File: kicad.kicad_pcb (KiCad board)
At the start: 2 copper layers, 100 x 70 mm, 65 parts, among them J1 Conn_01x03, J2 Screw_Terminal_01x02, J3 Conn_01x05, J4 jack3.5mm, J5 Screw_Terminal_01x02, J6 ICSP, J7 Screw_Terminal_01x03, J8 Screw_Terminal_01x03, K1 RELAY 0510, K2 RELAY 0510, Q1 BC817, Q2 BC817, SW1 SW_Push, SW2 SW_Push, T1 ZMPT101B, U1 KF33BD-TR, U2 ADS1015IDGS, U3 ESP-12E

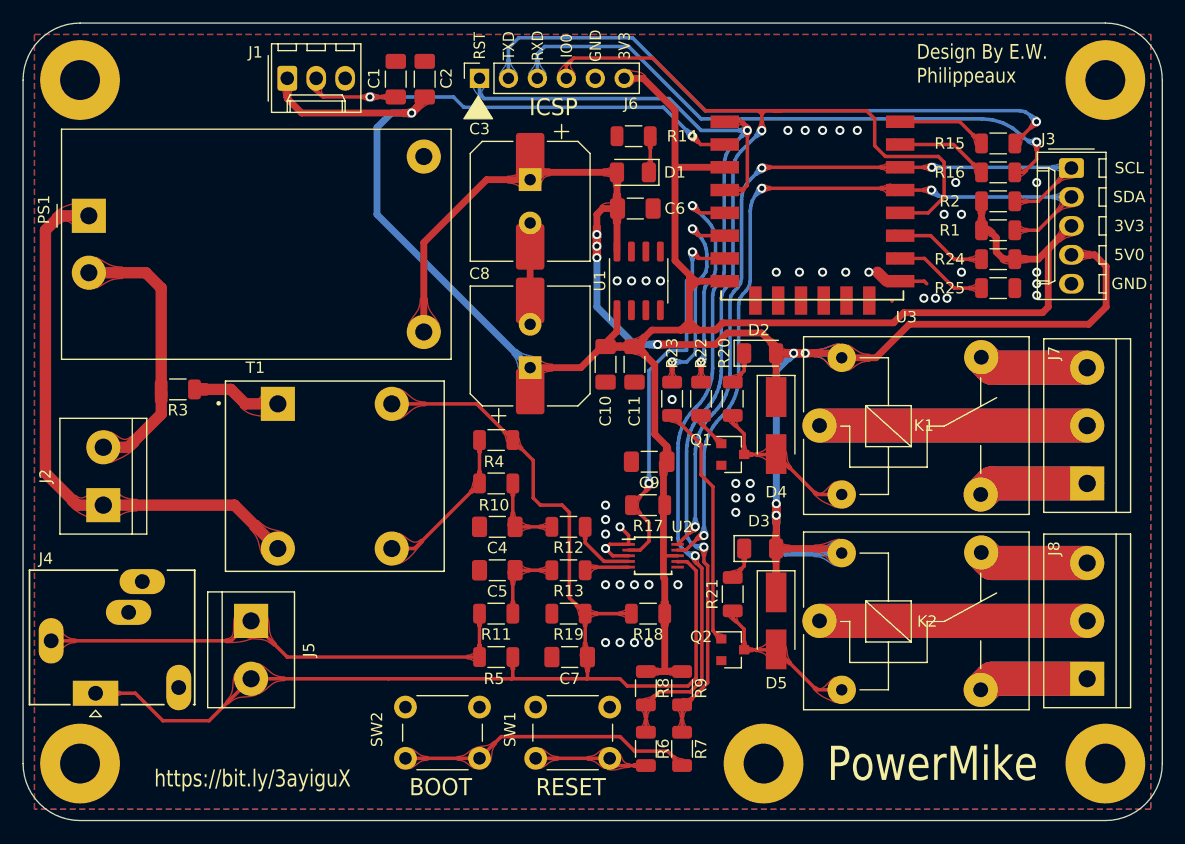
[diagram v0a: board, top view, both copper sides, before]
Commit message: Gerber exportado a .ZIP para JLCPCB
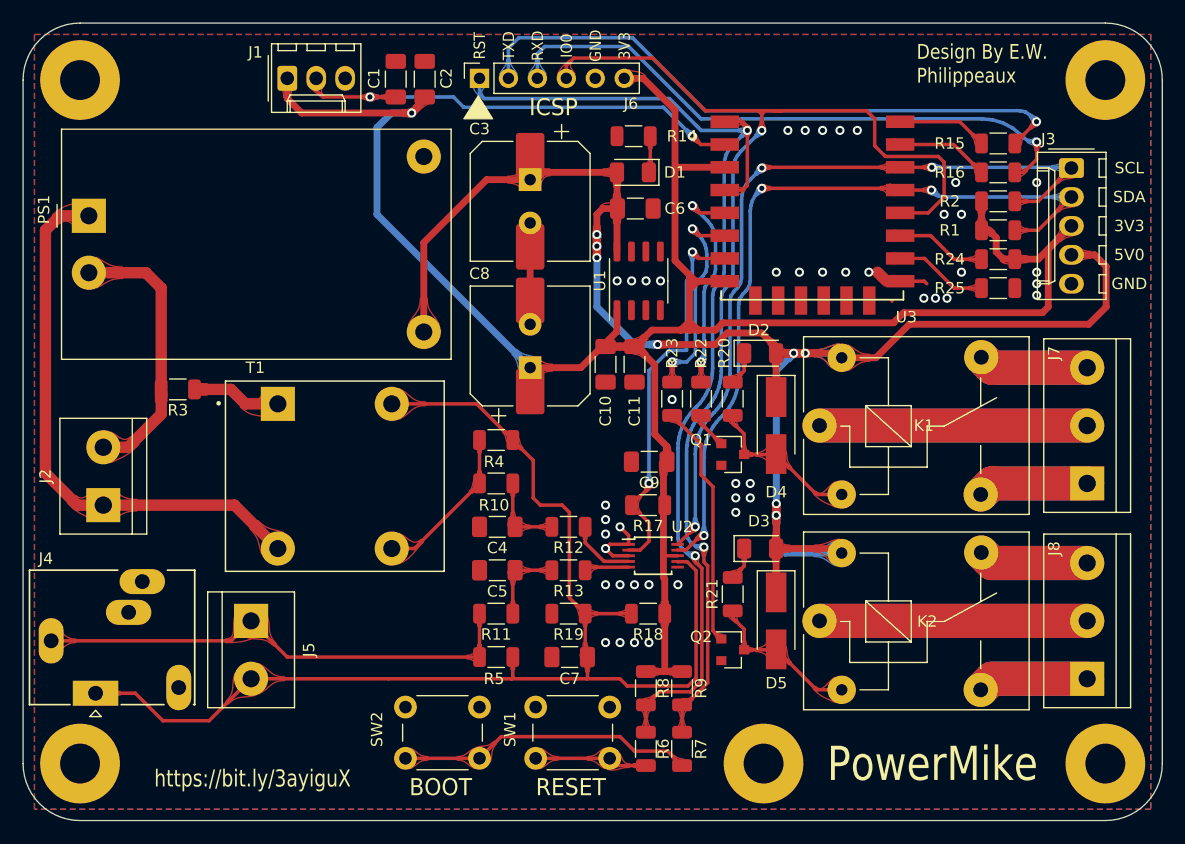
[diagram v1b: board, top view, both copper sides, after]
